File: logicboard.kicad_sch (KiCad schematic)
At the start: 41 parts, among them J1 USB_C_Receptacle_USB2.0, J2 Conn_01x04_Pin, U1 STM32F405RGT7, U2 USBLC6-2P6, U3 TJA1051T-3, U4 AMS1117-3.3, U6 LM22676QTJ-5.0, Y1 Crystal

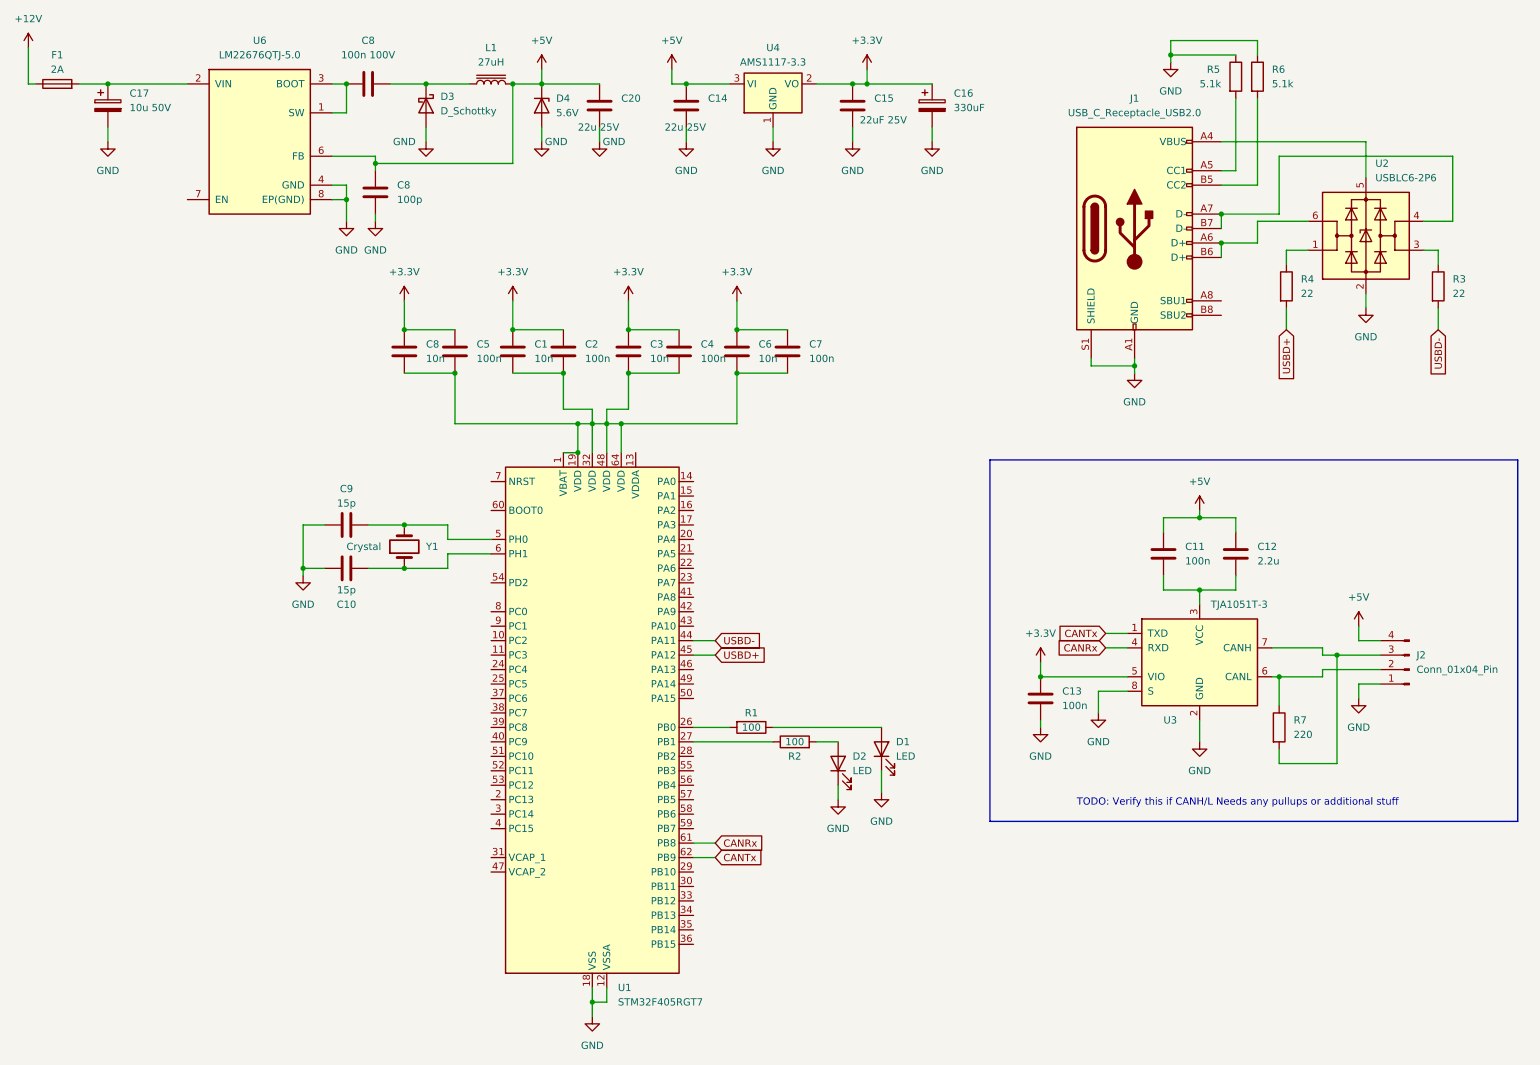
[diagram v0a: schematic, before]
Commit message: initial
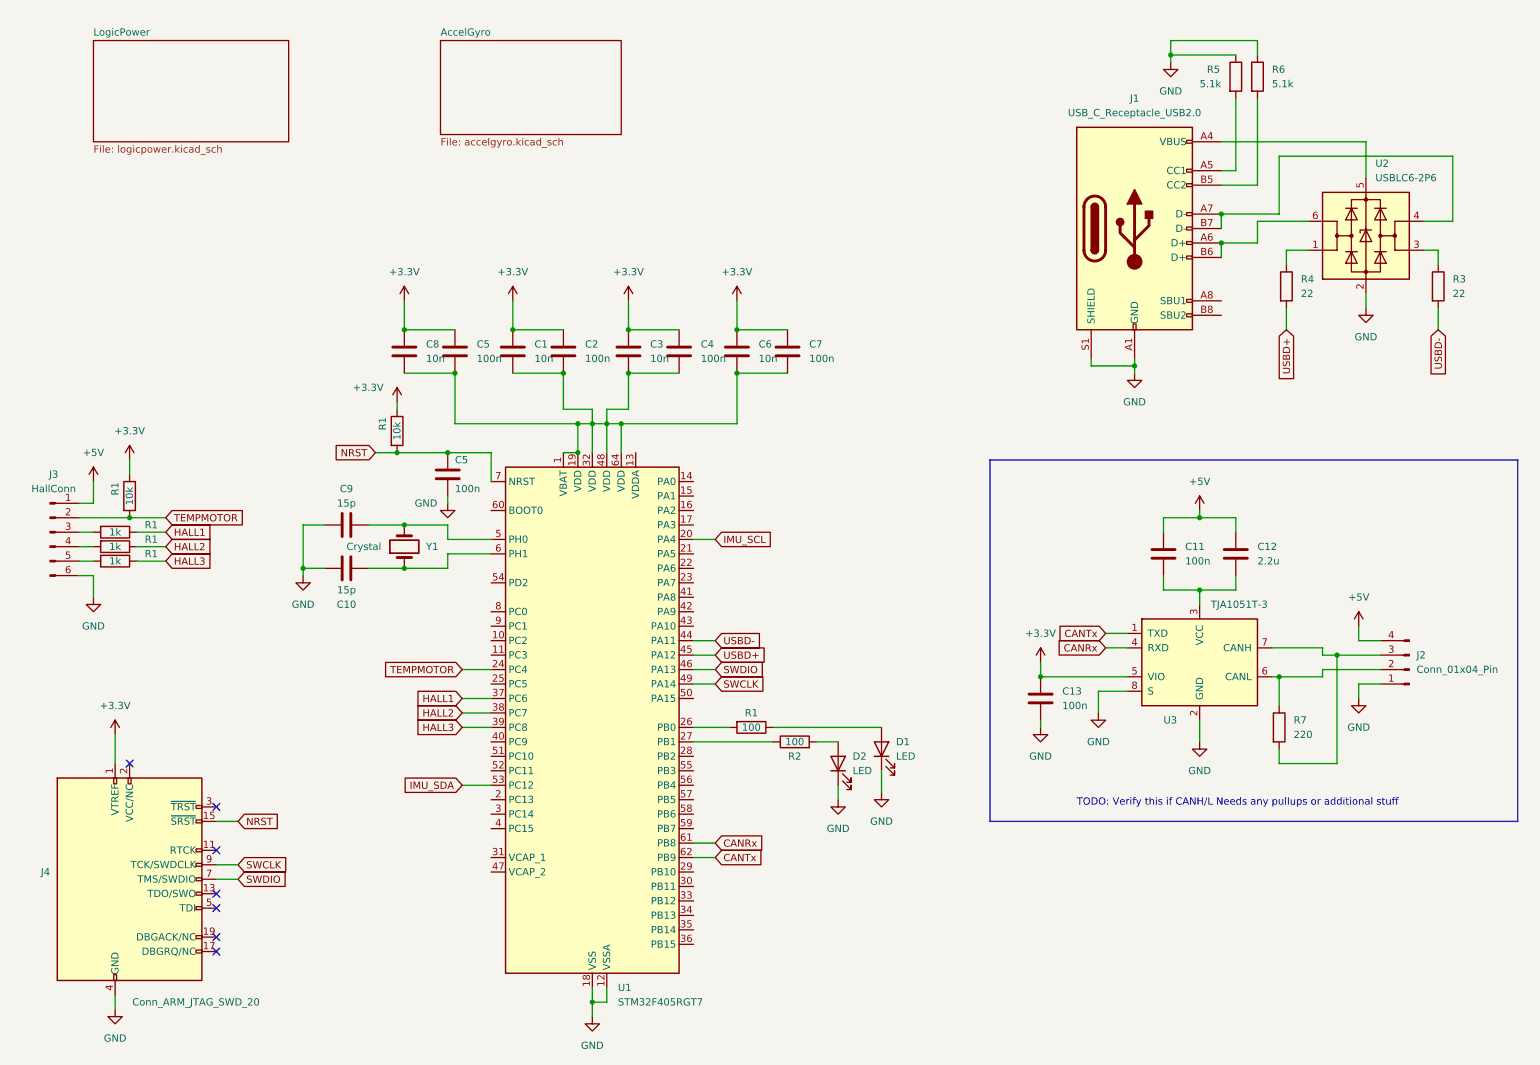
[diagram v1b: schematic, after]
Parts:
- removed C14, C20: 22u 25V, symbol Device:C
- removed C15: 22uF 25V, symbol Device:C
- removed C16: 330uF, symbol Device:C_Polarized
- removed C17: 10u 50V, symbol Device:C_Polarized
- removed C8: 100n 100V, symbol Device:C
- removed C8: 100p, symbol Device:C
- removed D3: D_Schottky, symbol Device:D_Schottky
- removed D4: 5.6V, symbol Device:D_Zener
- removed F1: 2A, symbol Device:Fuse
- removed L1: 27uH, symbol Device:L_Iron
- removed U4: AMS1117-3.3, Package_TO_SOT_SMD:SOT-223-3_TabPin2, symbol Regulator_Linear:AMS1117-3.3
- removed U6: LM22676QTJ-5.0, manuf:TO-263-7-TEXAS, symbol Schlib-texas:LM22676QTJ-5.0
- added C5: 100n, symbol Device:C
- added J3: HallConn, symbol Connector:Conn_01x06_Pin
- added J4: Conn_ARM_JTAG_SWD_20, symbol Connector:Conn_ARM_JTAG_SWD_20
- added R1 (x3): 1k, symbol Device:R
- added R1 (x2): 10k, symbol Device:R
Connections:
- net +3.3V: now also J4.1 (VTREF), R1.1, R1.1
- net +5V: now also J3.1 (Pin_1)
- net GND: now also C5.2, J3.6 (Pin_6), J4.10 (GND), J4.12 (GND), J4.14 (GND), J4.16 (GND), J4.18 (GND), J4.20 (GND), J4.4 (GND), J4.6 (GND), J4.8 (GND)
- net IMU_SCL: now reaches U1.20 (PA4)
- net TEMPMOTOR: now reaches U1.24 (PC4)
- net TEMPMOTOR: now also J3.2 (Pin_2), R1.2
- net HALL1: now reaches U1.37 (PC6)
- net HALL1: now also R1.1
- net HALL2: now reaches U1.38 (PC7)
- net HALL2: now also R1.1
- net HALL3: now reaches U1.39 (PC8)
- net HALL3: now also R1.1
- net SWDIO: now reaches U1.46 (PA13)
- net SWDIO: now also J4.7 (TMS/SWDIO)
- net SWCLK: now reaches U1.49 (PA14)
- net SWCLK: now also J4.9 (TCK/SWDCLK)
- net IMU_SDA: now reaches U1.53 (PC12)
- net NRST: now reaches U1.7 (NRST)
- net NRST: now also C5.1, J4.15 (~{SRST}), R1.2
- new net: J3.3 (Pin_3), R1.2
- new net: J3.4 (Pin_4), R1.2
- new net: J3.5 (Pin_5), R1.2
- no-connect marks 0 -> 7
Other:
- added sheet AccelGyro (accelgyro.kicad_sch)
- added sheet LogicPower (logicpower.kicad_sch)

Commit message: initial
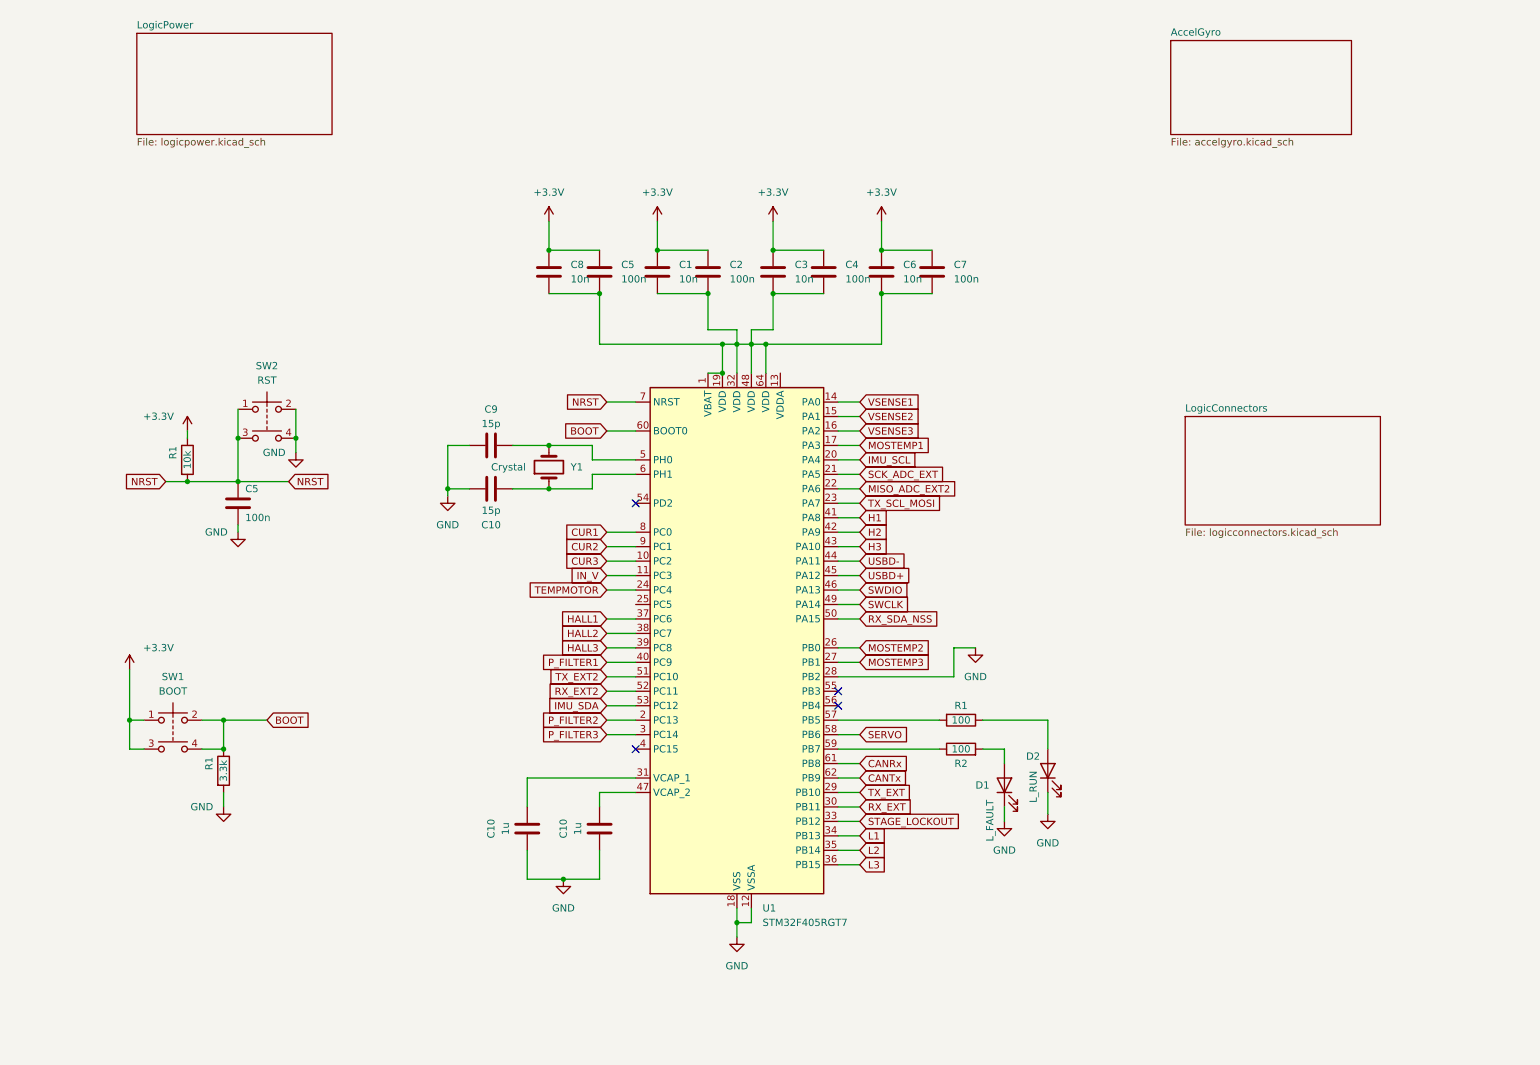
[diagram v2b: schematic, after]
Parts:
- removed C11, C13: 100n, symbol Device:C
- removed C12: 2.2u, symbol Device:C
- removed J1: USB_C_Receptacle_USB2.0, symbol Connector:USB_C_Receptacle_USB2.0
- removed J2: Conn_01x04_Pin, symbol Connector:Conn_01x04_Pin
- removed J3: HallConn, symbol Connector:Conn_01x06_Pin
- removed J4: Conn_ARM_JTAG_SWD_20, symbol Connector:Conn_ARM_JTAG_SWD_20
- removed R1 (x3): 1k, symbol Device:R
- removed R1: 10k, symbol Device:R
- removed R3, R4: 22, symbol Device:R
- removed R5, R6: 5.1k, symbol Device:R
- removed R7: 220, symbol Device:R
- removed U2: USBLC6-2P6, Package_TO_SOT_SMD:SOT-666, symbol Power_Protection:USBLC6-2P6
- removed U3: TJA1051T-3, Package_SO:SOIC-8_3.9x4.9mm_P1.27mm, symbol Interface_CAN_LIN:TJA1051T-3
- added C10 (x2): 1u, symbol Device:C
- added R1: 3.3k, symbol Device:R
- added SW1: BOOT, symbol Switch:SW_Push_Dual
- added SW2: RST, symbol Switch:SW_Push_Dual
- D1: value LED -> L_FAULT
- D2: value LED -> L_RUN
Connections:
- net +3.3V: now also SW1.1, SW1.3
- net GND: now also U1.28 (PB2), C10.2, C10.2, R1.2, SW2.2, SW2.4
- net NRST: now also SW2.1, SW2.3
- net at D1.2 (A): now also R2.2; no longer R1.1
- net at D2.2 (A): now also R1.1; no longer R2.2
- net at R2.1: now also U1.59 (PB7); no longer U1.27 (PB1)
- net CUR3: now reaches U1.10 (PC2)
- net IN_V: now reaches U1.11 (PC3)
- net VSENSE1: now reaches U1.14 (PA0)
- net VSENSE2: now reaches U1.15 (PA1)
- net VSENSE3: now reaches U1.16 (PA2)
- net MOSTEMP1: now reaches U1.17 (PA3)
- net P_FILTER2: now reaches U1.2 (PC13)
- net SCK_ADC_EXT: now reaches U1.21 (PA5)
- net MISO_ADC_EXT2: now reaches U1.22 (PA6)
- net TX_SCL_MOSI: now reaches U1.23 (PA7)
- net at R1.2: now also U1.57 (PB5); no longer U1.26 (PB0)
- net TX_EXT: now reaches U1.29 (PB10)
- net P_FILTER3: now reaches U1.3 (PC14)
- net RX_EXT: now reaches U1.30 (PB11)
- net at U1.31 (VCAP_1): now also C10.1
- net STAGE_LOCKOUT: now reaches U1.33 (PB12)
- net L1: now reaches U1.34 (PB13)
- net L2: now reaches U1.35 (PB14)
- net L3: now reaches U1.36 (PB15)
- net P_FILTER1: now reaches U1.40 (PC9)
- net H1: now reaches U1.41 (PA8)
- net H2: now reaches U1.42 (PA9)
- net H3: now reaches U1.43 (PA10)
- net at U1.47 (VCAP_2): now also C10.1
- net RX_SDA_NSS: now reaches U1.50 (PA15)
- net TX_EXT2: now reaches U1.51 (PC10)
- net RX_EXT2: now reaches U1.52 (PC11)
- net SERVO: now reaches U1.58 (PB6)
- net BOOT: now reaches U1.60 (BOOT0)
- net BOOT: now also R1.1, SW1.2, SW1.4
- net CUR1: now reaches U1.8 (PC0)
- net CUR2: now reaches U1.9 (PC1)
- new net MOSTEMP2: U1.26 (PB0)
- new net MOSTEMP3: U1.27 (PB1)
- no-connect marks 7 -> 4
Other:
- added sheet LogicConnectors (logicconnectors.kicad_sch)
- note removed: "TODO: Verify this if CANH/L Needs any pullups or additional stuff"
- moved on the sheet: C1, C10, C2, C3, C4, C5, C6, C7, C8, C9, D1, D2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

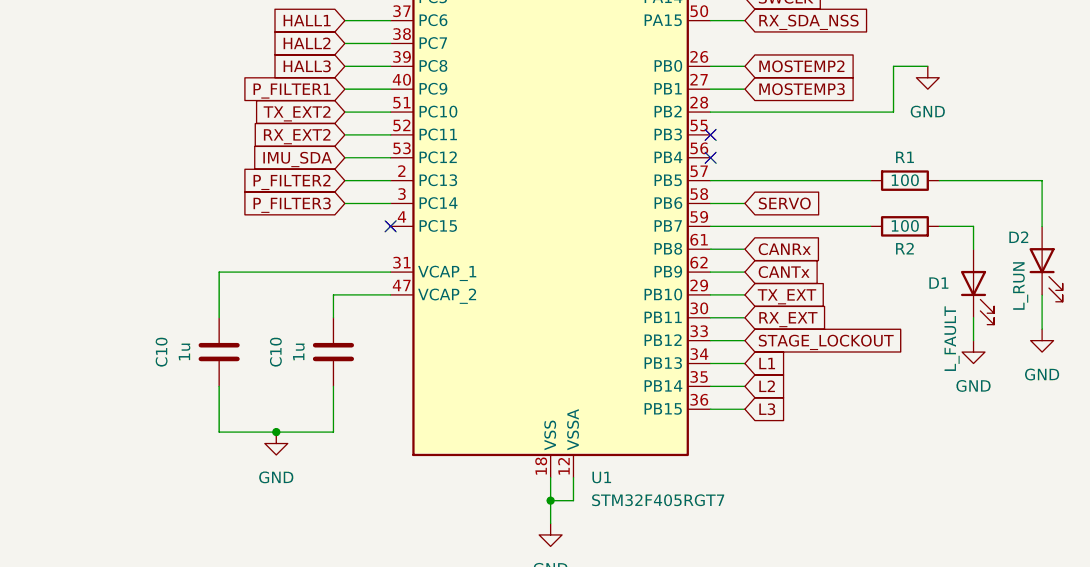
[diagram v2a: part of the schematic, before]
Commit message: drivers
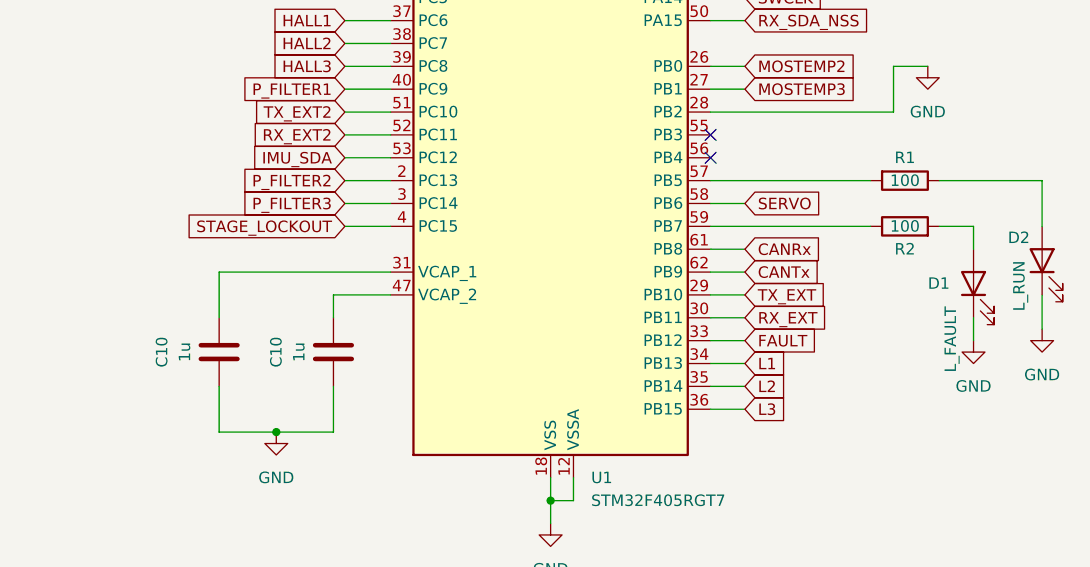
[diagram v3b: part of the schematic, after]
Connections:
- net STAGE_LOCKOUT: now also U1.4 (PC15); no longer U1.33 (PB12)
- new net FAULT: U1.33 (PB12)
- no-connect marks 4 -> 3
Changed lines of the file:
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@@
   )
   (no_connect (at 160.02 135.89))
-  (no_connect (at 124.46 146.05))
   (no_connect (at 160.02 138.43))
   (no_connect (at 124.46 102.87))
@@
     (stroke (width 0) (type default))
   )
+  (wire (pts (xy 119.38 146.05) (xy 124.46 146.05))
+    (stroke (width 0) (type default))
+  )
   (wire (pts (xy 160.02 158.75) (xy 163.83 158.75))
     (stroke (width 0) (type default))
@@
     )
   )
-  (global_label "STAGE_LOCKOUT" (shape input) (at 163.83 158.75 0) (fields_autoplaced)
-    (effects (font (size 1.27 1.27)) (justify left))
-    (property "Intersheetrefs" "${INTERSHEET_REFS}" (at 181.2611 158.75 0)
-      (effects (font (size 1.27 1.27)) (justify left) hide)
+  (global_label "STAGE_LOCKOUT" (shape input) (at 119.38 146.05 180) (fields_autoplaced)
+    (effects (font (size 1.27 1.27)) (justify right))
+    (property "Intersheetrefs" "${INTERSHEET_REFS}" (at 101.9489 146.05 0)
+      (effects (font (size 1.27 1.27)) (justify right) hide)
     )
   )
@@
       (effects (font (size 1.27 1.27)) (justify left) hide)
     )
+  )
+  (global_label "FAULT" (shape input) (at 163.83 158.75 0) (fields_autoplaced)
+    (effects (font (size 1.27 1.27)) (justify left))
+    (property "Intersheetrefs" "${INTERSHEET_REFS}" (at 171.585 158.75 0)
+      (effects (font (size 1.27 1.27)) (justify left) hide)
+    )
